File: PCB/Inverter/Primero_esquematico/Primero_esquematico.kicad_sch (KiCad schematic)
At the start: 0 parts

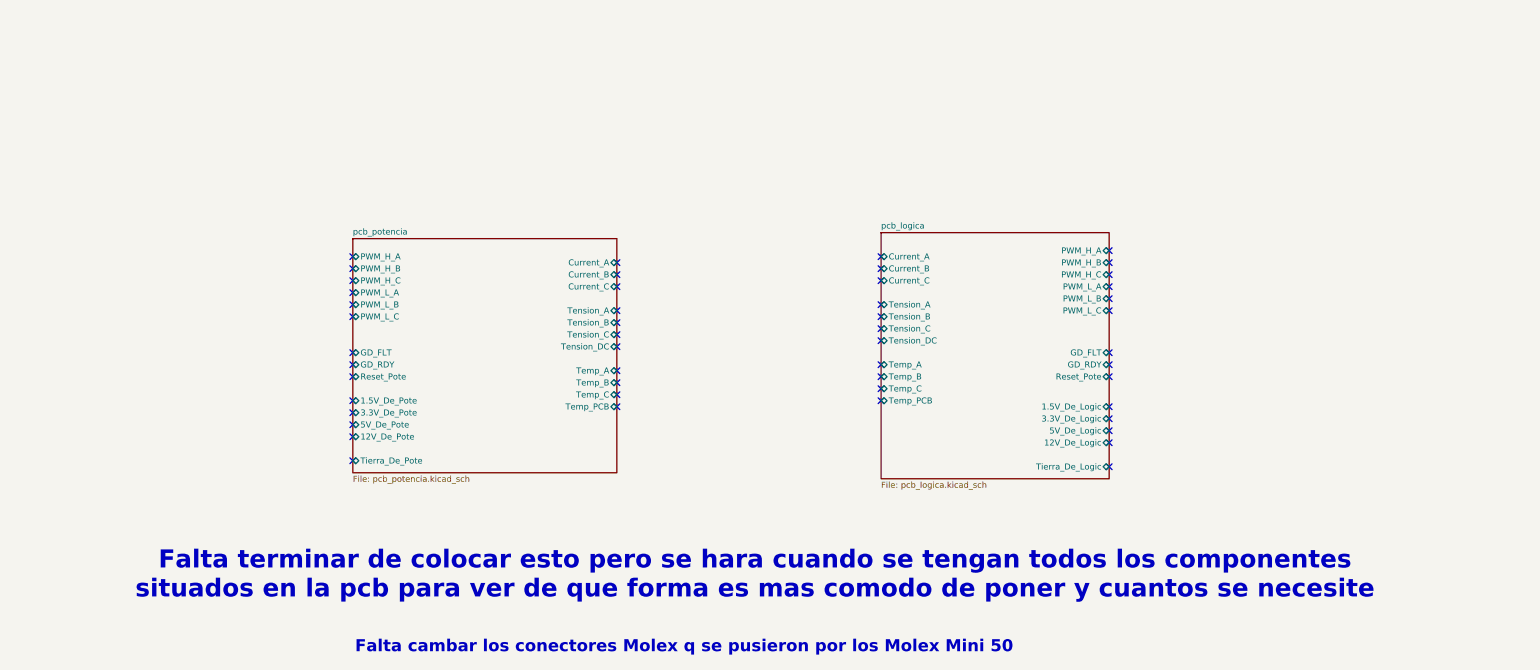
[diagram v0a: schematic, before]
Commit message: Algunos cambios
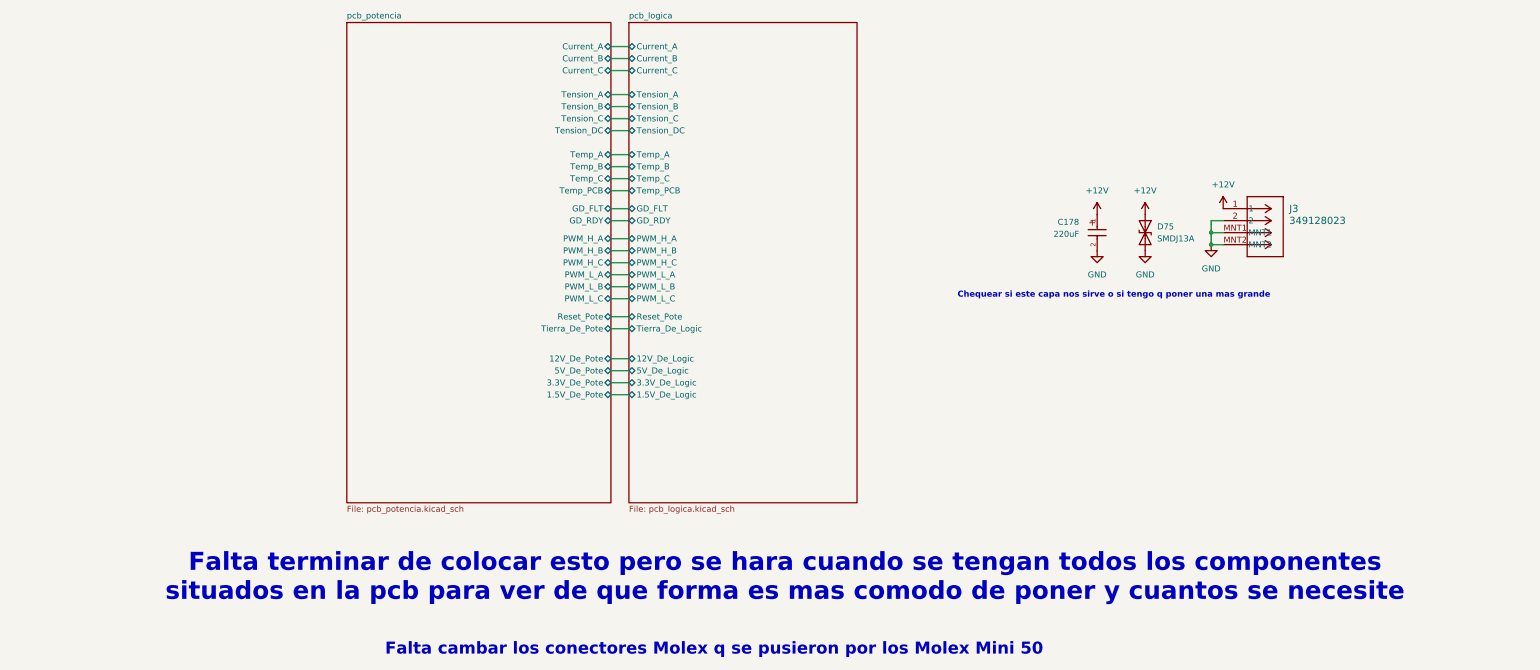
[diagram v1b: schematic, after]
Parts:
- added C178: 220uF, Snapeda:WCAP-PSLC_8X11.7_DXL_, symbol Snapeda:WCAP-PSLC_8X11.7
- added D75: SMDJ13A, Diode_SMD:D_SMC, symbol Device:D_TVS
- added J3: 349128023, Snapeda:CONN_SD-34912-001_02_MOL, symbol Snapeda:349128023
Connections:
- new net +12V: C178.1, D75.1 (A1), J3.1
- new net GND: C178.2, D75.2 (A2), J3.2, J3.MNT1, J3.MNT2
- no-connect marks 50 -> 0
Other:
- note added: "Chequear si este capa nos sirve o si tengo q poner una mas grande"
